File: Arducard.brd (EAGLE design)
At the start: 90 x 50 mm, 19 parts, among them U1 ATMEGA328P, U2 MPR121V2, U3 TPS61097-33DBVR, Y1 8MHZ

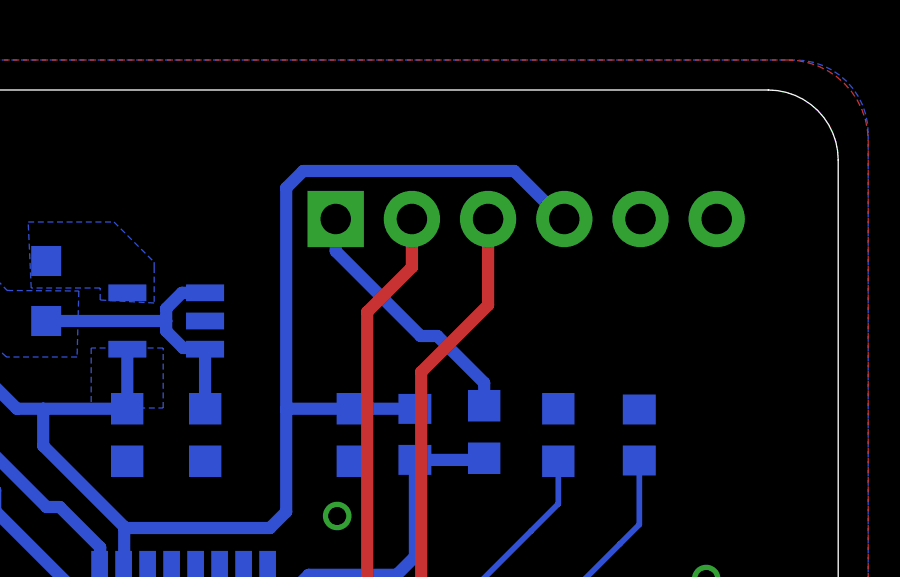
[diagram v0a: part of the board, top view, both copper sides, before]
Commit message: Arducard Board (Eagle)
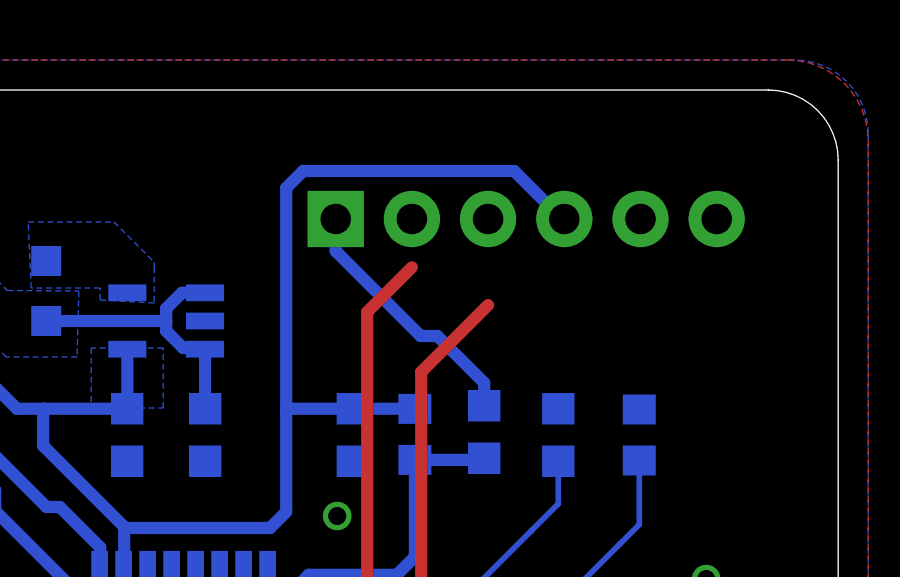
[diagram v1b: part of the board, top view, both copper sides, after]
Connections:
- net RX: now also JP1.P$3; no longer JP1.P$2
- net TX: now also JP1.P$2; no longer JP1.P$3
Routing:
- net TX: track 22.1 -> 19.3 mm
- net RX: track 19.1 -> 17.4 mm
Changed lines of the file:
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@@
 </signal>
 <signal name="RX">
-<contactref element="JP1" pad="P$2"/>
 <contactref element="U1" pad="30"/>
 <wire x1="72.4726" y1="28.51" x2="73.31" y2="28.51" width="0.4064" layer="16"/>
@@
 <wire x1="74.3" y1="29.5" x2="74.3" y2="42.6" width="0.4064" layer="1"/>
 <wire x1="74.3" y1="42.6" x2="75.79" y2="44.09" width="0.4064" layer="1"/>
-<wire x1="75.79" y1="44.09" x2="75.79" y2="45.7" width="0.4064" layer="1"/>
+<contactref element="JP1" pad="P$3"/>
+<wire x1="75.79" y1="44.09" x2="78.33" y2="45.7" width="0" layer="19" extent="1-1"/>
 </signal>
 <signal name="TX">
-<contactref element="JP1" pad="P$3"/>
 <contactref element="U1" pad="31"/>
 <wire x1="72.4726" y1="27.71" x2="75.31" y2="27.71" width="0.4064" layer="16"/>
@@
 <wire x1="76.1" y1="28.4" x2="76.1" y2="40.6" width="0.4064" layer="1"/>
 <wire x1="76.1" y1="40.6" x2="78.33" y2="42.83" width="0.4064" layer="1"/>
-<wire x1="78.33" y1="42.83" x2="78.33" y2="45.7" width="0.4064" layer="1"/>
+<contactref element="JP1" pad="P$2"/>
+<wire x1="78.33" y1="42.83" x2="75.79" y2="45.7" width="0" layer="19" extent="1-1"/>
 </signal>
 </signals>

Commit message: Arducard Board (Eagle)
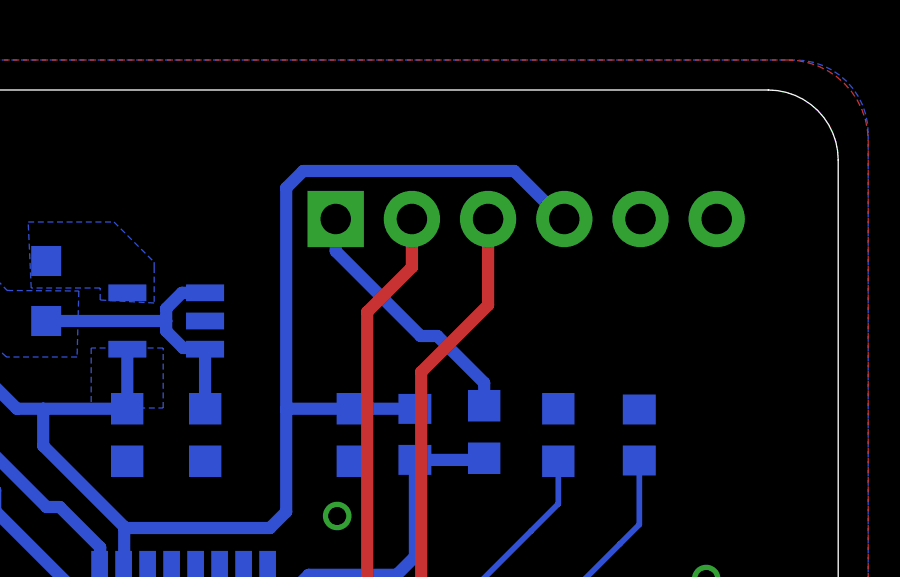
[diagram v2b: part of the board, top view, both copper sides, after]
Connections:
- net RX: now also JP1.P$2; no longer JP1.P$3
- net TX: now also JP1.P$3; no longer JP1.P$2
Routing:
- net TX: track 19.3 -> 22.1 mm
- net RX: track 17.4 -> 19.1 mm
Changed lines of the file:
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@@
 </signal>
 <signal name="RX">
+<contactref element="JP1" pad="P$2"/>
 <contactref element="U1" pad="30"/>
 <wire x1="72.4726" y1="28.51" x2="73.31" y2="28.51" width="0.4064" layer="16"/>
@@
 <wire x1="74.3" y1="29.5" x2="74.3" y2="42.6" width="0.4064" layer="1"/>
 <wire x1="74.3" y1="42.6" x2="75.79" y2="44.09" width="0.4064" layer="1"/>
-<contactref element="JP1" pad="P$3"/>
-<wire x1="75.79" y1="44.09" x2="78.33" y2="45.7" width="0" layer="19" extent="1-1"/>
+<wire x1="75.79" y1="44.09" x2="75.79" y2="45.7" width="0.4064" layer="1"/>
 </signal>
 <signal name="TX">
+<contactref element="JP1" pad="P$3"/>
 <contactref element="U1" pad="31"/>
 <wire x1="72.4726" y1="27.71" x2="75.31" y2="27.71" width="0.4064" layer="16"/>
@@
 <wire x1="76.1" y1="28.4" x2="76.1" y2="40.6" width="0.4064" layer="1"/>
 <wire x1="76.1" y1="40.6" x2="78.33" y2="42.83" width="0.4064" layer="1"/>
-<contactref element="JP1" pad="P$2"/>
-<wire x1="78.33" y1="42.83" x2="75.79" y2="45.7" width="0" layer="19" extent="1-1"/>
+<wire x1="78.33" y1="42.83" x2="78.33" y2="45.7" width="0.4064" layer="1"/>
 </signal>
 </signals>
